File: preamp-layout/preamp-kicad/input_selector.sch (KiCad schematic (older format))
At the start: 45 parts, among them J35 Conn_01x03_Male, J36 Conn_01x03_Male, J37 Conn_01x03_Male, J38 Conn_01x03_Male, J39 Conn_01x03_Male, J40 Conn_01x03_Male, J41 Conn_01x03_Male, J42 Conn_01x03_Female, J43 Conn_01x03_Female, J44 Conn_01x02_Female, J45 Conn_01x07_Female, J46 Conn_01x07_Female, J47 Conn_01x02_Male, J48 Conn_01x02_Male, K2 G6JU, K3 G6JU, K4 G6JU, K5 G6JU, K6 G6JU, K7 G6JU, K8 G6JU, U10 ULN2003, U8 MCP23017_SO, U9 ULN2003

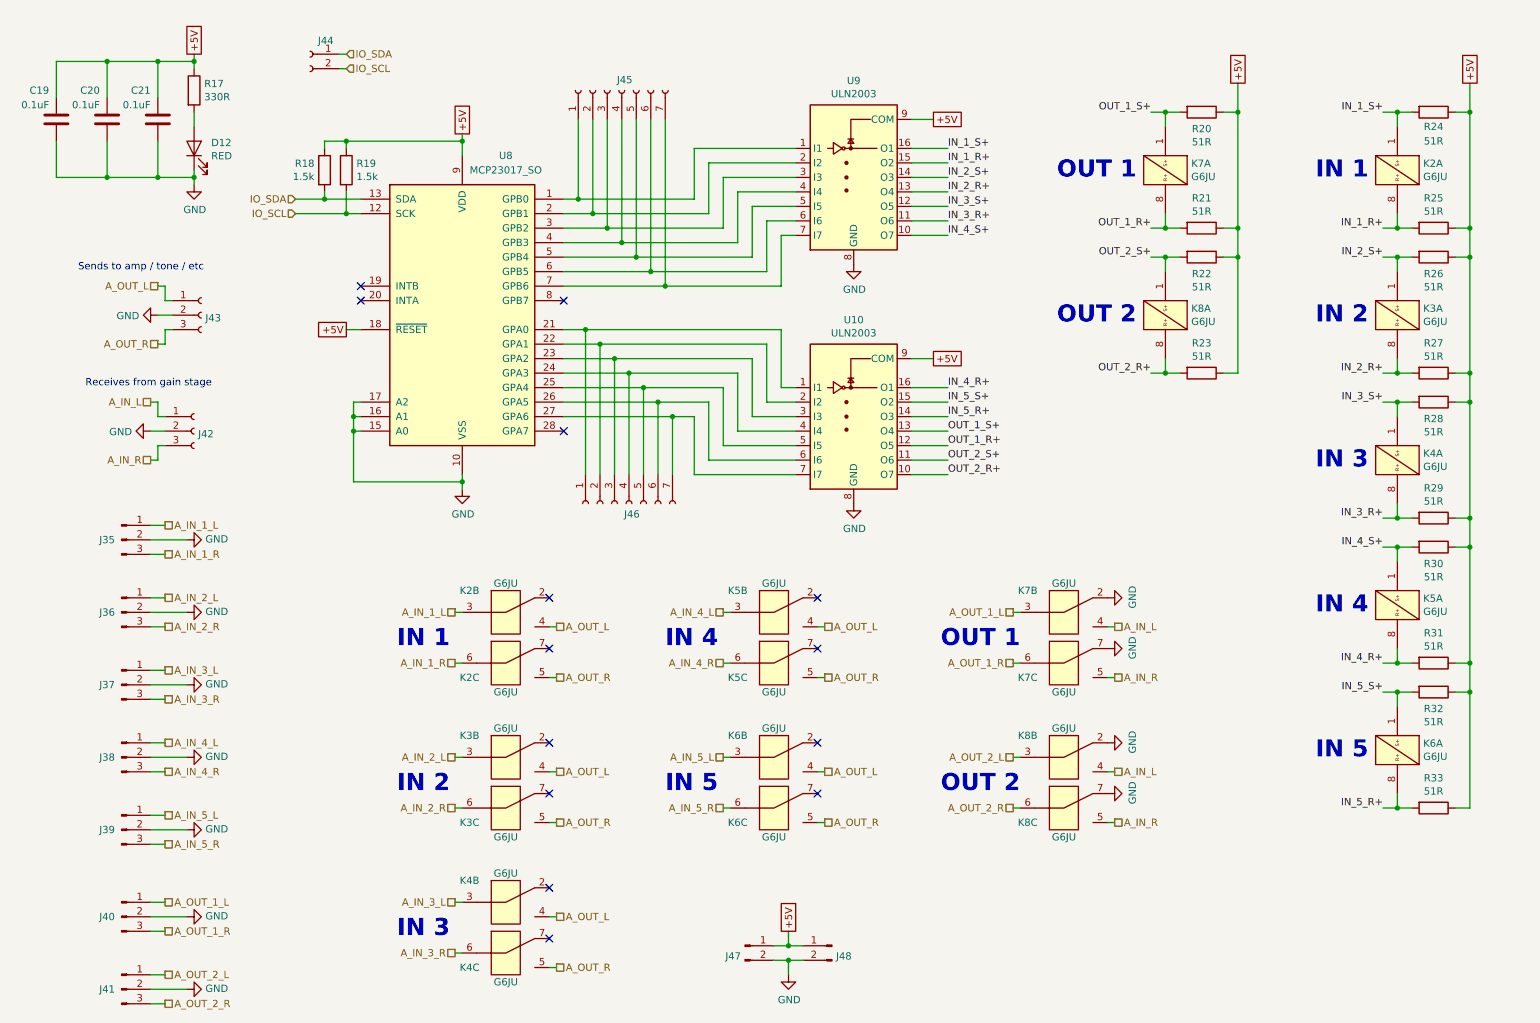
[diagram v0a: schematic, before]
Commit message: Periodic backup
Extensive changes as a result of PCB layout phase.
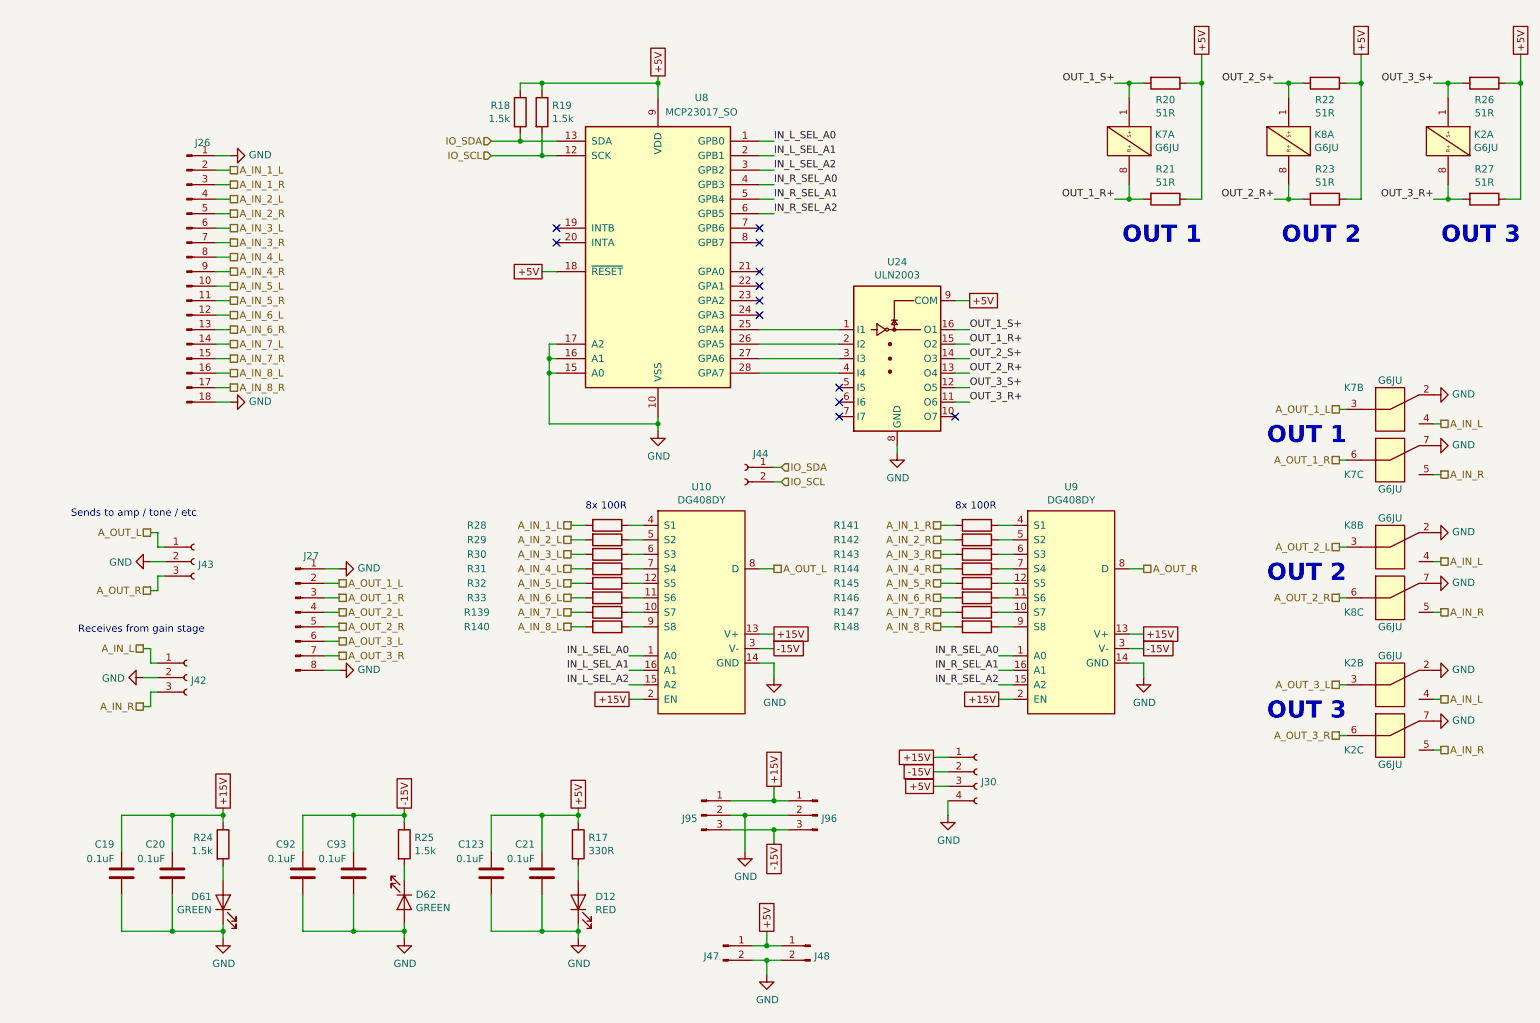
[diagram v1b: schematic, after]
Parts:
- removed J35, J36, J37, J38, J39, J40, J41: Conn_01x03_Male, Connector_PinHeader_2.54mm:PinHeader_1x03_P2.54mm_Vertical, symbol Connector:Conn_01x03_Male
- removed J45, J46: Conn_01x07_Female, Connector_PinHeader_2.54mm:PinHeader_1x07_P2.54mm_Vertical, symbol Connector:Conn_01x07_Female
- removed K3, K4, K5, K6: G6JU, preamp:Relay_DPDT_Omron_G6JU-2P-Y, symbol preamp:G6JU
- removed U10, U9: ULN2003, Package_SO:SOIC-16_3.9x9.9mm_P1.27mm, symbol Transistor_Array:ULN2003
- added C123, C92, C93: 0.1uF, Capacitor_SMD:C_0805_2012Metric_Pad1.15x1.40mm_HandSolder, symbol Device:C
- added D61, D62: GREEN, LED_SMD:LED_1206_3216Metric_Pad1.42x1.75mm_HandSolder, symbol Device:LED
- added J26: Conn_01x18_Male, Connector_PinHeader_2.54mm:PinHeader_1x18_P2.54mm_Vertical, symbol Connector:Conn_01x18_Male
- added J27: Conn_01x08_Male, Connector_PinHeader_2.54mm:PinHeader_1x08_P2.54mm_Vertical, symbol Connector:Conn_01x08_Male
- added J30: Conn_01x04_Female, Connector_PinSocket_2.54mm:PinSocket_1x04_P2.54mm_Vertical, symbol Connector:Conn_01x04_Female
- added J95, J96: Conn_01x03_Male, Connector_JST:JST_EH_S3B-EH_1x03_P2.50mm_Horizontal, symbol Connector:Conn_01x03_Male
- added R139, R140, R141, R142, R143, R144, R145, R146, R147, R148: 100R, Resistor_SMD:R_1206_3216Metric_Pad1.42x1.75mm_HandSolder, symbol Device:R
- added U10, U9: DG408DY, Package_SO:SOIC-16_3.9x9.9mm_P1.27mm, symbol preamp:DG408DY
- added U24: ULN2003, Package_SO:SOIC-16_3.9x9.9mm_P1.27mm, symbol Transistor_Array:ULN2003
- J42, J43: footprint Connector_PinHeader_2.54mm:PinHeader_1x03_P2.54mm_Vertical -> Connector_PinSocket_2.54mm:PinSocket_1x03_P2.54mm_Vertical
- J44: footprint Connector_PinHeader_2.54mm:PinHeader_1x02_P2.54mm_Vertical -> Connector_JST:JST_EH_S2B-EH_1x02_P2.50mm_Horizontal
- J47, J48: footprint Connector_JST:JST_EH_B2B-EH-A_1x02_P2.50mm_Vertical -> Connector_JST:JST_EH_S2B-EH_1x02_P2.50mm_Horizontal
- R24, R25: value 51R -> 1.5k
- R28, R29, R30, R31, R32, R33: value 51R -> 100R
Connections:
- net IN_3_R+ is gone; now on net A_IN_2_L: R29.2
- net IN_3_S+ is gone; now on net A_IN_1_L: R28.2
- net IN_4_R+ is gone; now on net A_IN_4_L: R31.2
- net IN_4_S+ is gone; now on net A_IN_3_L: R30.2
- net IN_5_S+ is gone; now on net A_IN_5_L: R32.2
- net +5V: now also C123.1, J30.3 (Pin_3), U24.9 (COM); no longer C19.1, C20.1, R24.1, R25.1, R28.1, R29.1, R30.1, R31.1, R32.1, R33.1
- net A_IN_1_L: now also J26.2 (Pin_2); no longer K2.3
- net A_IN_1_R: now also J26.3 (Pin_3), R141.2; no longer K2.6
- net A_IN_2_L: now also J26.4 (Pin_4)
- net A_IN_2_R: now also J26.5 (Pin_5), R142.2
- net A_IN_3_L: now also J26.6 (Pin_6)
- net A_IN_3_R: now also J26.7 (Pin_7), R143.2
- net A_IN_4_L: now also J26.8 (Pin_8)
- net A_IN_4_R: now also J26.9 (Pin_9), R144.2
- net A_IN_5_L: now also J26.10 (Pin_10)
- net A_IN_5_R: now also J26.11 (Pin_11), R145.2
- net A_IN_L: now also K2.4
- net A_IN_R: now also K2.5
- net A_OUT_1_L: now also J27.2 (Pin_2)
- net A_OUT_1_R: now also J27.3 (Pin_3)
- net A_OUT_2_L: now also J27.4 (Pin_4)
- net A_OUT_2_R: now also J27.5 (Pin_5)
- net A_OUT_L: now also U10.8 (D); no longer K2.4
- net A_OUT_R: now also U9.8 (D); no longer K2.5
- net GND: now also K2.2, K2.7, C123.2, C92.2, C93.2, D61.1 (K), D62.2 (A), J26.1 (Pin_1), J26.18 (Pin_18), J27.1 (Pin_1), J27.8 (Pin_8), J30.4 (Pin_4), J95.2 (Pin_2), J96.2 (Pin_2), U10.14 (GND), U24.8 (GND), U9.14 (GND)
- net OUT_1_R+: now also U24.15 (O2)
- net OUT_1_S+: now also U24.16 (O1)
- net OUT_2_R+: now also U24.13 (O4)
- net OUT_2_S+: now also U24.14 (O3)
- net IN_L_SEL_A0: now reaches U8.1 (GPB0)
- net IN_L_SEL_A0: now also U10.1 (A0)
- net IN_L_SEL_A1: now reaches U8.2 (GPB1)
- net IN_L_SEL_A1: now also U10.16 (A1)
- net IN_L_SEL_A2: now reaches U8.3 (GPB2)
- net IN_L_SEL_A2: now also U10.15 (A2)
- net IN_R_SEL_A0: now reaches U8.4 (GPB3)
- net IN_R_SEL_A0: now also U9.1 (A0)
- net IN_R_SEL_A1: now reaches U8.5 (GPB4)
- net IN_R_SEL_A1: now also U9.16 (A1)
- net IN_R_SEL_A2: now reaches U8.6 (GPB5)
- net IN_R_SEL_A2: now also U9.15 (A2)
- net at U8.25 (GPA4): now also U24.1 (I1)
- net at U8.26 (GPA5): now also U24.2 (I2)
- net at U8.27 (GPA6): now also U24.3 (I3)
- net at U8.28 (GPA7): now also U24.4 (I4)
- net IN_1_R+: no longer names the net of R25.2
- net IN_1_R+: now also D62.1 (K); no longer K2.8
- net IN_1_S+: no longer names the net of R24.2
- net IN_1_S+: now also D61.2 (A); no longer K2.1
- net IN_2_R+ renamed OUT_3_R+
- net OUT_3_R+: now also K2.8, U24.11 (O6)
- net IN_2_S+ renamed OUT_3_S+
- net OUT_3_S+: now also K2.1, U24.12 (O5)
- net IN_5_R+ renamed A_IN_6_L
- net A_IN_6_L: now also J26.12 (Pin_12)
- new net: R139.1, U10.10 (S7)
- new net: R33.1, U10.11 (S6)
- new net: R32.1, U10.12 (S5)
- new net: R28.1, U10.4 (S1)
- new net: R29.1, U10.5 (S2)
- new net: R30.1, U10.6 (S3)
- new net: R31.1, U10.7 (S4)
- new net: R140.1, U10.9 (S8)
- new net: R147.1, U9.10 (S7)
- new net: R146.1, U9.11 (S6)
- new net: R145.1, U9.12 (S5)
- new net: R141.1, U9.4 (S1)
- new net: R142.1, U9.5 (S2)
- new net: R143.1, U9.6 (S3)
- new net: R144.1, U9.7 (S4)
- new net: R148.1, U9.9 (S8)
- new net +15V: C19.1, C20.1, J30.1 (Pin_1), J95.1 (Pin_1), J96.1 (Pin_1), R24.1, U10.13 (V+), U10.2 (EN), U9.13 (V+), U9.2 (EN)
- new net -15V: C92.1, C93.1, J30.2 (Pin_2), J95.3 (Pin_3), J96.3 (Pin_3), R25.1, U10.3 (V-), U9.3 (V-)
- new net A_IN_6_R: J26.13 (Pin_13), R146.2
- new net A_IN_7_L: J26.14 (Pin_14), R139.2
- new net A_IN_7_R: J26.15 (Pin_15), R147.2
- new net A_IN_8_L: J26.16 (Pin_16), R140.2
- new net A_IN_8_R: J26.17 (Pin_17), R148.2
- new net A_OUT_3_L: J27.6 (Pin_6), K2.3
- new net A_OUT_3_R: J27.7 (Pin_7), K2.6
- no-connect marks 14 -> 12
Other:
- note added: "8x 100R"
- note added: "OUT 3"
- note removed: "IN 1"
- note removed: "IN 2"
- note removed: "IN 3"
- note removed: "IN 4"
- note removed: "IN 5"
- moved on the sheet: C19, C20, C21, D12, J42, J43, J44, J47, J48, K7A, K7B, K7C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
